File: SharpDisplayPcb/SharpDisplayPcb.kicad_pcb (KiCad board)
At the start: 2 copper layers, 53.2 x 52.4 mm, 2 parts

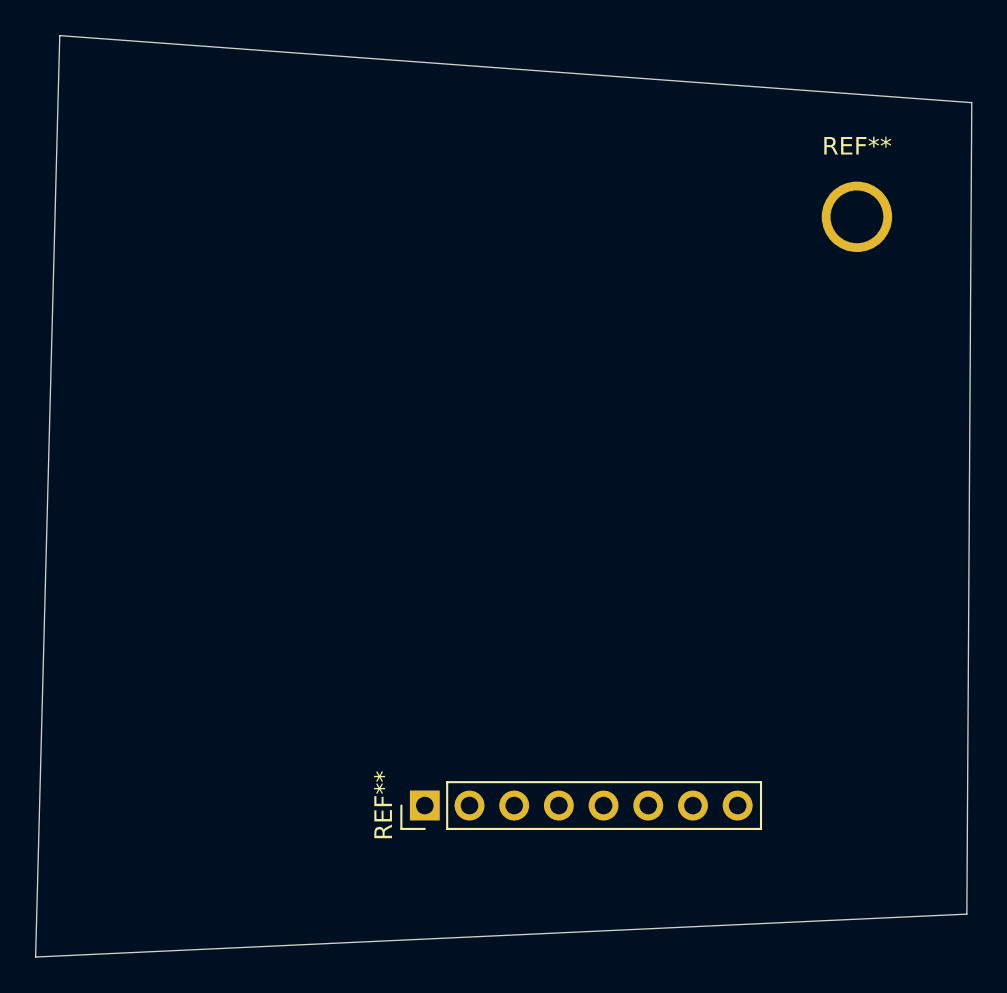
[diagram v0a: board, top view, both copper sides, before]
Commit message: PCB border, start schematic
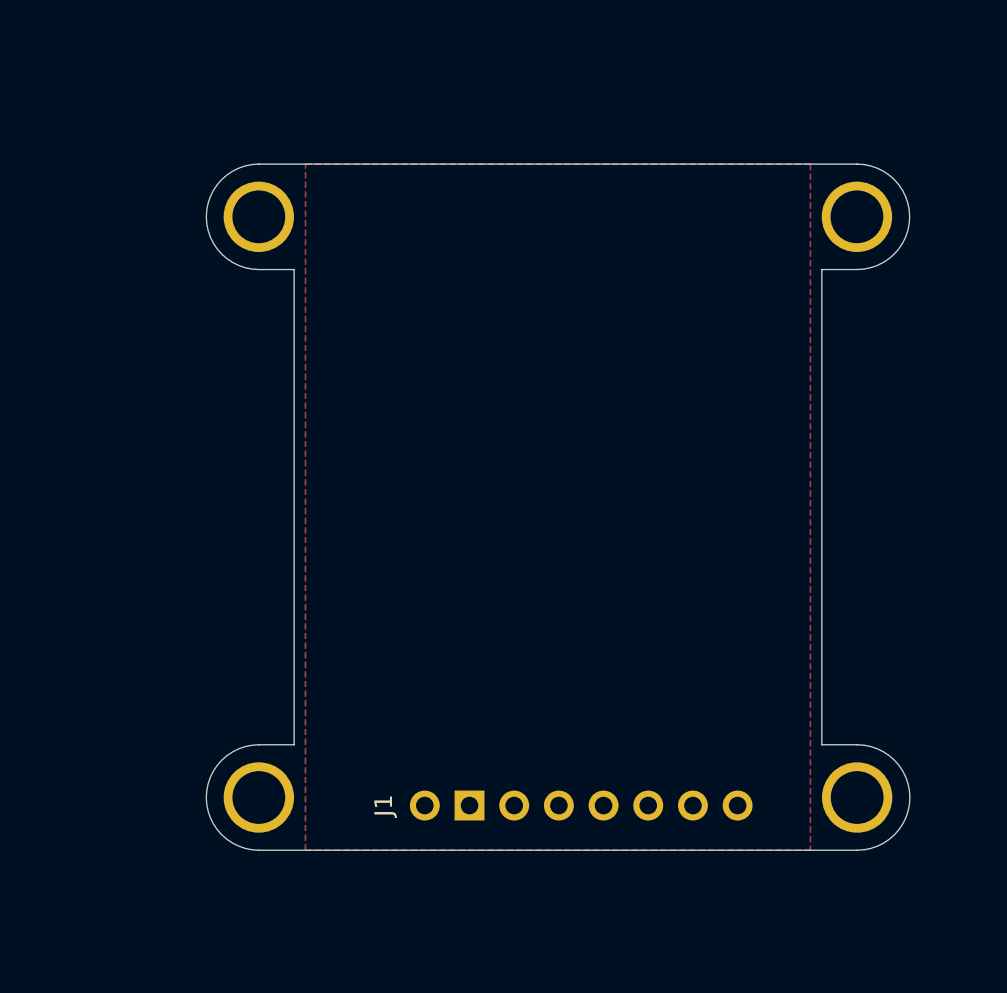
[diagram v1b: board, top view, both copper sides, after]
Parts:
- removed REF**: PinHeader_1x08_P2.54mm_Vertical, Connector_PinHeader_2.54mm:PinHeader_1x08_P2.54mm_Vertical
- added J1: Conn_01x08_Female, Connector_PinHeader_2.54mm:PinHeader_1x08_P2.54mm_Vertical, F.Cu at (100.0, 103.9)
- added M3: MH3, MountingHole:MountingHole_3mm_Pad, F.Cu at (124.6, 103.4)
- added M3: MH3, MountingHole:MountingHole_3mm_Pad, F.Cu at (90.6, 103.4)
- added M3: MH3, MountingHole:MountingHole_3mm_Pad, F.Cu at (90.6, 70.4)
- M3: renamed from REF**; value MountingHole_3mm_Pad -> MH3
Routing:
- added copper zone on B.Cu, net GND
- added copper zone on F.Cu, net GND
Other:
- board size 53.2 x 52.4 mm -> 40 x 39 mm
